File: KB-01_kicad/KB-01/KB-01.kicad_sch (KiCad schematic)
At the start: 0 parts

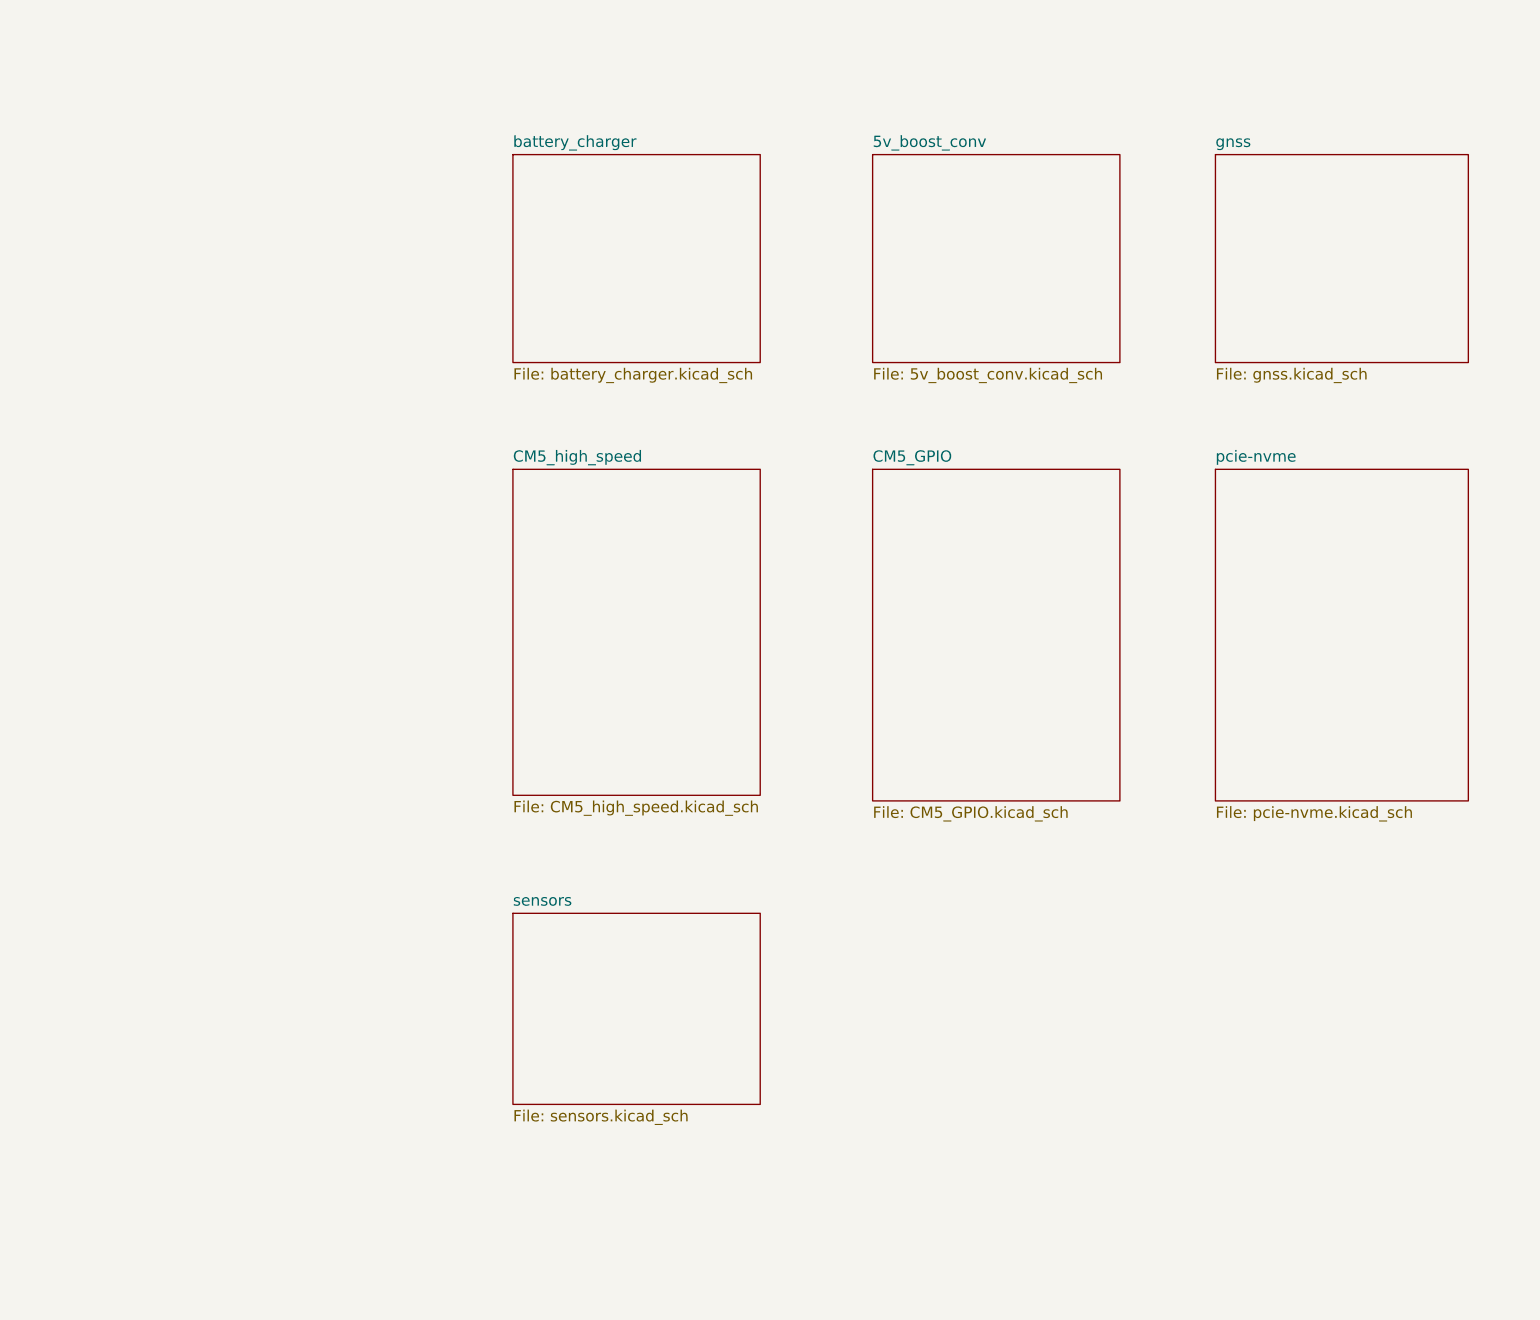
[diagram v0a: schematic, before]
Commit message: up
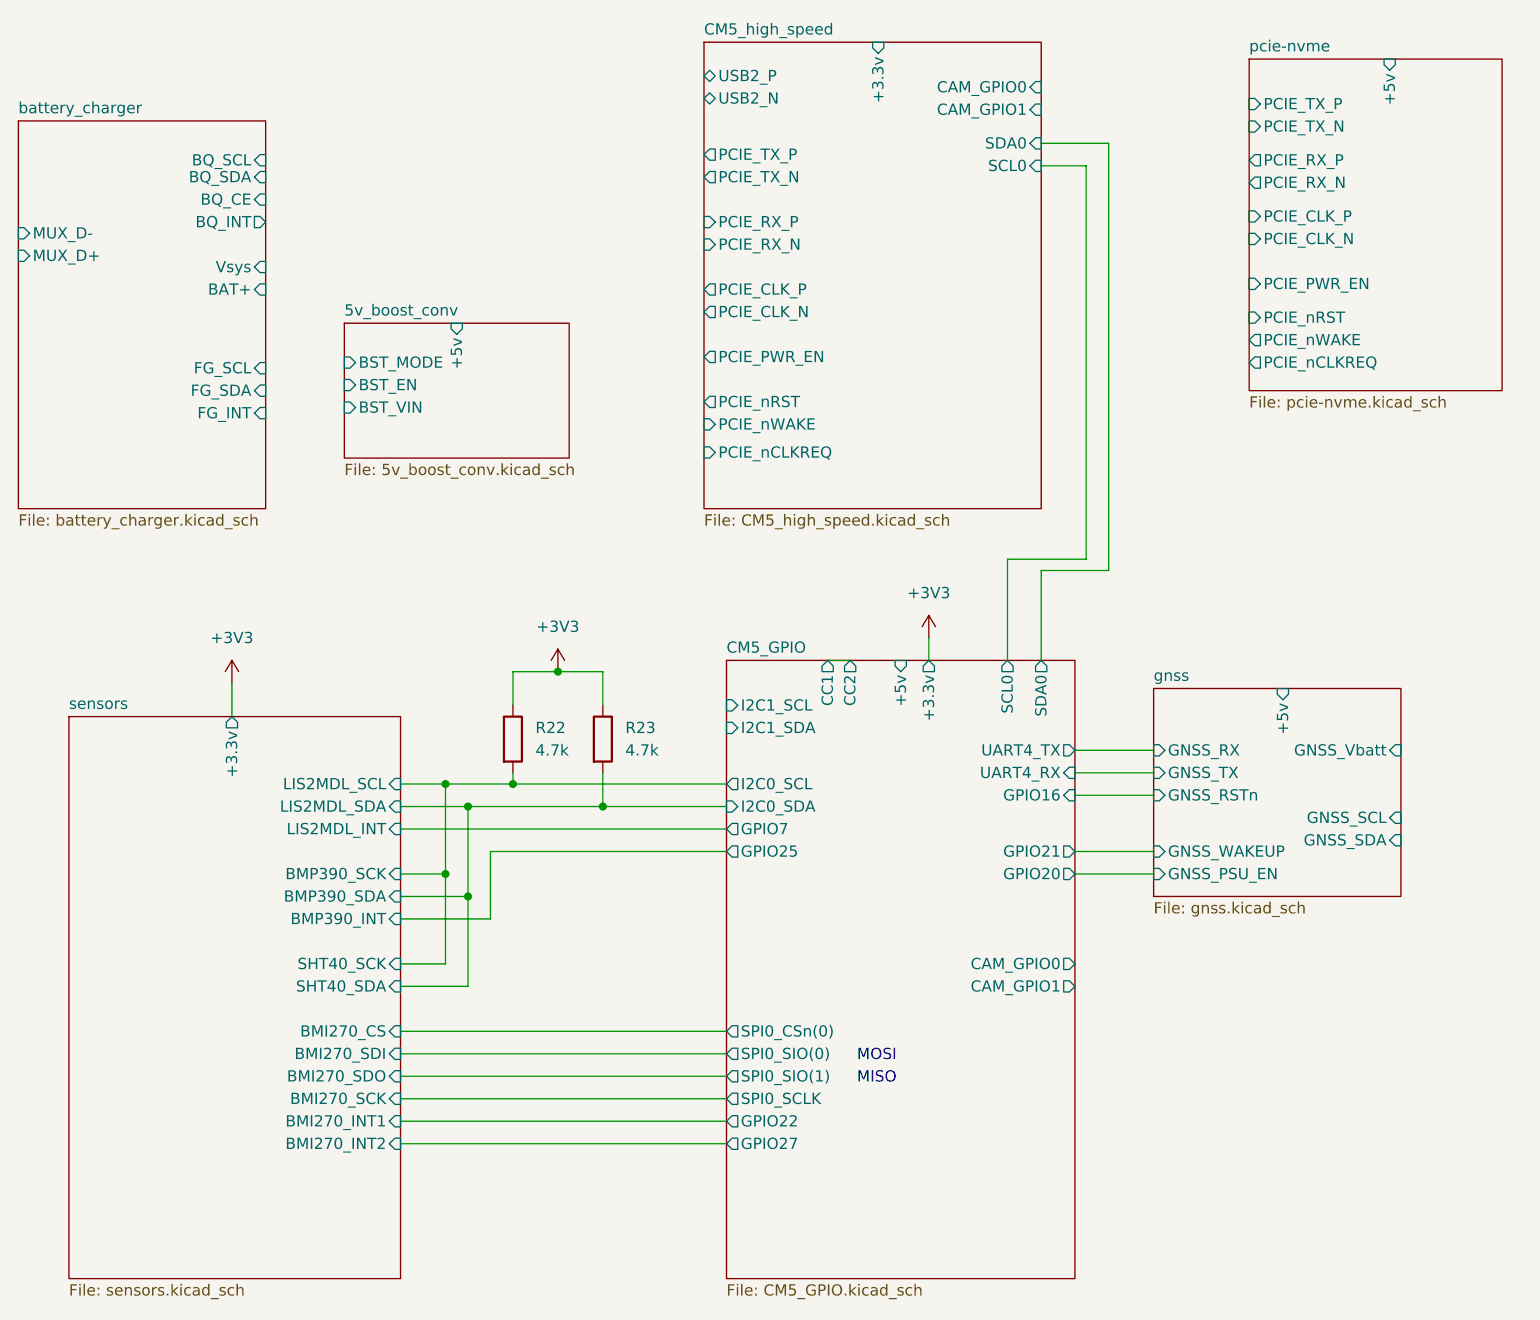
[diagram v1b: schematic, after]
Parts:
- added R22, R23: 4.7k, symbol Device:R
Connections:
- new net +3V3: R22.1, R23.1
- new net CM5_GPIO/I2C0_SCL: R22.2
- new net CM5_GPIO/I2C0_SDA: R23.2
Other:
- sheet 5v_boost_conv ports: added +5v, BST_EN, BST_MODE, BST_VIN; removed none
- sheet CM5_GPIO ports: added +3.3v, +5v, CAM_GPIO0, CAM_GPIO1, CC1, CC2, GPIO16, GPIO20, GPIO21, GPIO22, GPIO25, GPIO27, GPIO7, I2C0_SCL, I2C0_SDA, I2C1_SCL, I2C1_SDA, SCL0, SDA0, SPI0_CSn(0), SPI0_SCLK, SPI0_SIO(0), SPI0_SIO(1), UART4_RX, UART4_TX; removed none
- sheet CM5_high_speed ports: added +3.3v, CAM_GPIO0, CAM_GPIO1, PCIE_CLK_N, PCIE_CLK_P, PCIE_PWR_EN, PCIE_RX_N, PCIE_RX_P, PCIE_TX_N, PCIE_TX_P, PCIE_nCLKREQ, PCIE_nRST, PCIE_nWAKE, SCL0, SDA0, USB2_N, USB2_P; removed none
- sheet battery_charger ports: added BAT+, BQ_CE, BQ_INT, BQ_SCL, BQ_SDA, FG_INT, FG_SCL, FG_SDA, MUX_D+, MUX_D-, Vsys; removed none
- sheet gnss ports: added +5v, GNSS_PSU_EN, GNSS_RSTn, GNSS_RX, GNSS_SCL, GNSS_SDA, GNSS_TX, GNSS_Vbatt, GNSS_WAKEUP; removed none
- sheet pcie-nvme ports: added +5v, PCIE_CLK_N, PCIE_CLK_P, PCIE_PWR_EN, PCIE_RX_N, PCIE_RX_P, PCIE_TX_N, PCIE_TX_P, PCIE_nCLKREQ, PCIE_nRST, PCIE_nWAKE; removed none
- sheet sensors ports: added +3.3v, BMI270_CS, BMI270_INT1, BMI270_INT2, BMI270_SCK, BMI270_SDI, BMI270_SDO, BMP390_INT, BMP390_SCK, BMP390_SDA, LIS2MDL_INT, LIS2MDL_SCL, LIS2MDL_SDA, SHT40_SCK, SHT40_SDA; removed none
- note added: "MISO"
- note added: "MOSI"
